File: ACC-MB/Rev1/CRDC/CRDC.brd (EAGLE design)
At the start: 180 x 64 mm, 7 parts

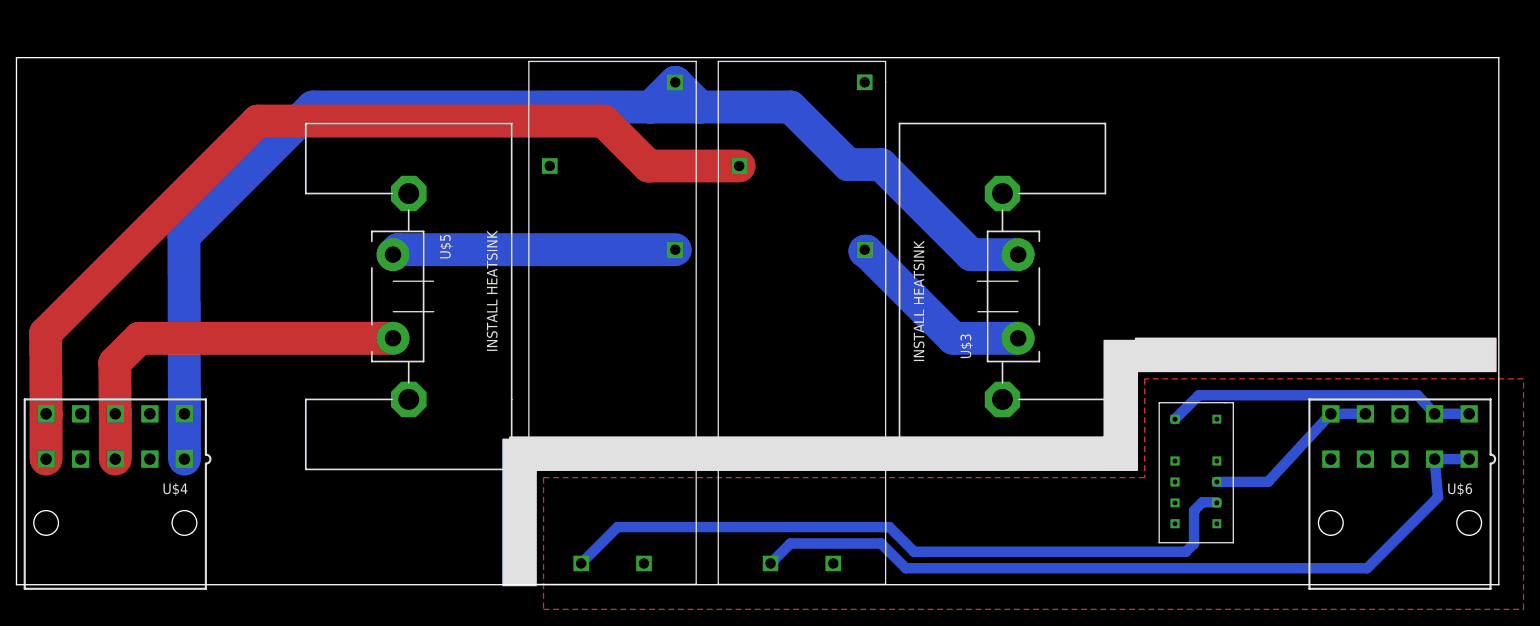
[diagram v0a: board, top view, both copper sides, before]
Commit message: update
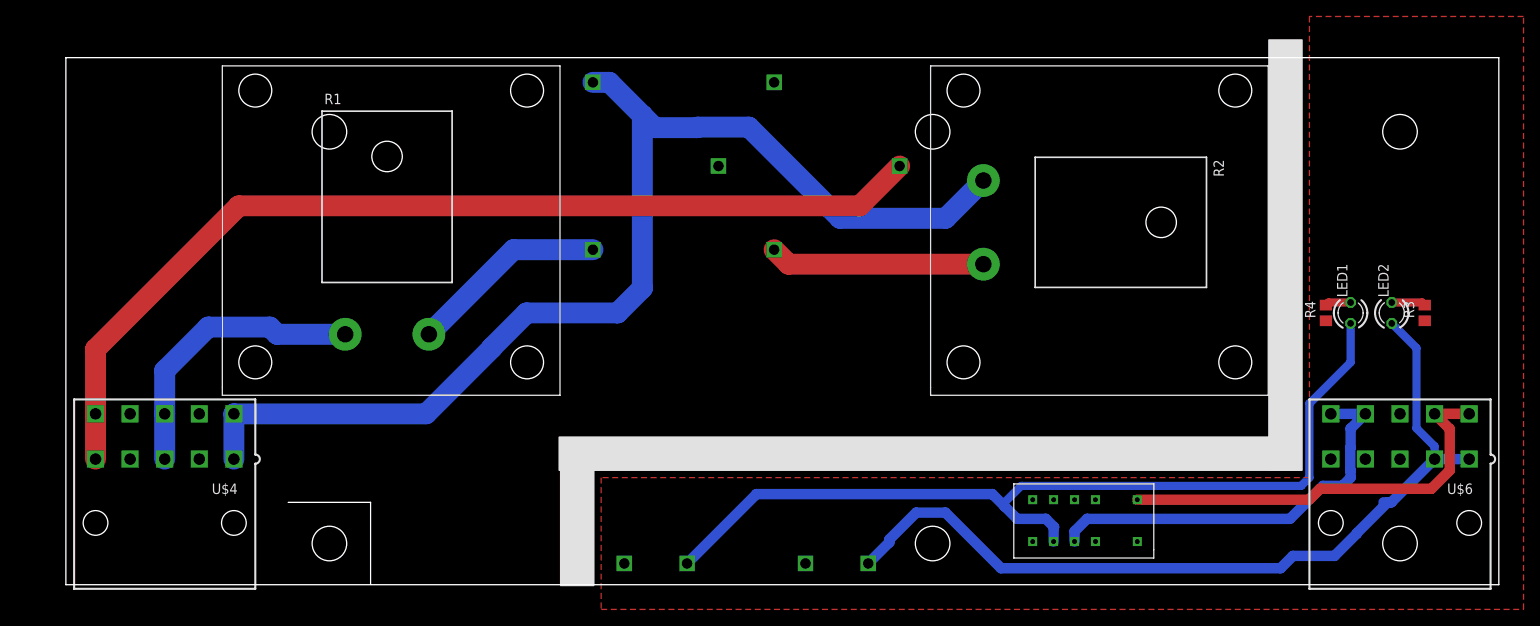
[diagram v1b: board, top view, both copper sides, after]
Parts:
- removed U$5: TO247RESISTORHEATINK, ACC-MB-R0:_CUSTOM_TO-247-2V
- added LED1, LED2: (no value), ACC-MB-R0:LED3MM
- added R1, R2: (no value), ACC-MB-R0:TO-247-2H
- added R3, R4: (no value), ACC-MB-R0:R0805
- added U$8, U$9: HEATSINK40X40X15, ACC-MB-R0:HEATSINK40X40X15
- U$3: value TO247RESISTORHEATINK -> BENDER_IRR155; device ACC-MB-R0:_CUSTOM_TO-247-2V -> ACC-MB-R0:BENDER_IRR155
- moved U$3 90.3 mm to (50.0, 60.0), flipped to the bottom, turned to 180 degrees
- moved U$7 17.7 mm to (153.1, 5.24), turned to 180 degrees
- moved U$2 11.0 mm to (109.0, 61.0), flipped to the bottom
- moved U$1 10.0 mm to (87.0, 61.0), flipped to the bottom
- moved U$4 6.00 mm to (35.0, 18.0)
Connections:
- net HV-_DRY renamed HV-_DRY_AUX
- new net N$1: LED2.K, R3.2
- new net N$5: LED1.K, R4.2
- net DISCHARGE: now also LED2.A
- net GND: now also R3.1, R4.1
- net HV+_DRY: now also R2.1; no longer U$3.2
- net HV+_WET: now also R1.1; no longer U$5.2
- net N$21: now also R1.2; no longer U$5.1
- net N$4: now also R2.2; no longer U$3.1
- net PRECHARGE: now also LED1.A
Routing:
- net +12V: track 21.7 -> 50.2 mm
- net PRECHARGE: track 85.1 -> 111.0 mm
- net PRECHARGE_SIG: track 37.9 -> 51.2 mm
- net HV+_DRY: track 150.8 -> 138.6 mm
- net HV+_WET: track 46.7 -> 35.2 mm
- net N$21: track 34.5 -> 24.2 mm
- net HV-_DRY_AUX: track 112.4 -> 120.2 mm
- net DISCHARGE: track 95.7 -> 103.2 mm
- net N$1: track 0.00 -> 4.13 mm
- net N$5: track 0.00 -> 3.13 mm
- net N$4: track 23.0 -> 26.1 mm
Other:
- board size 180 x 64 mm -> 174 x 64 mm
